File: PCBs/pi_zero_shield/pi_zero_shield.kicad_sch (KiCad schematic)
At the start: 4 parts, among them J1 T1M-10-F-SH-L-K, J3 T1M-06-X-DV

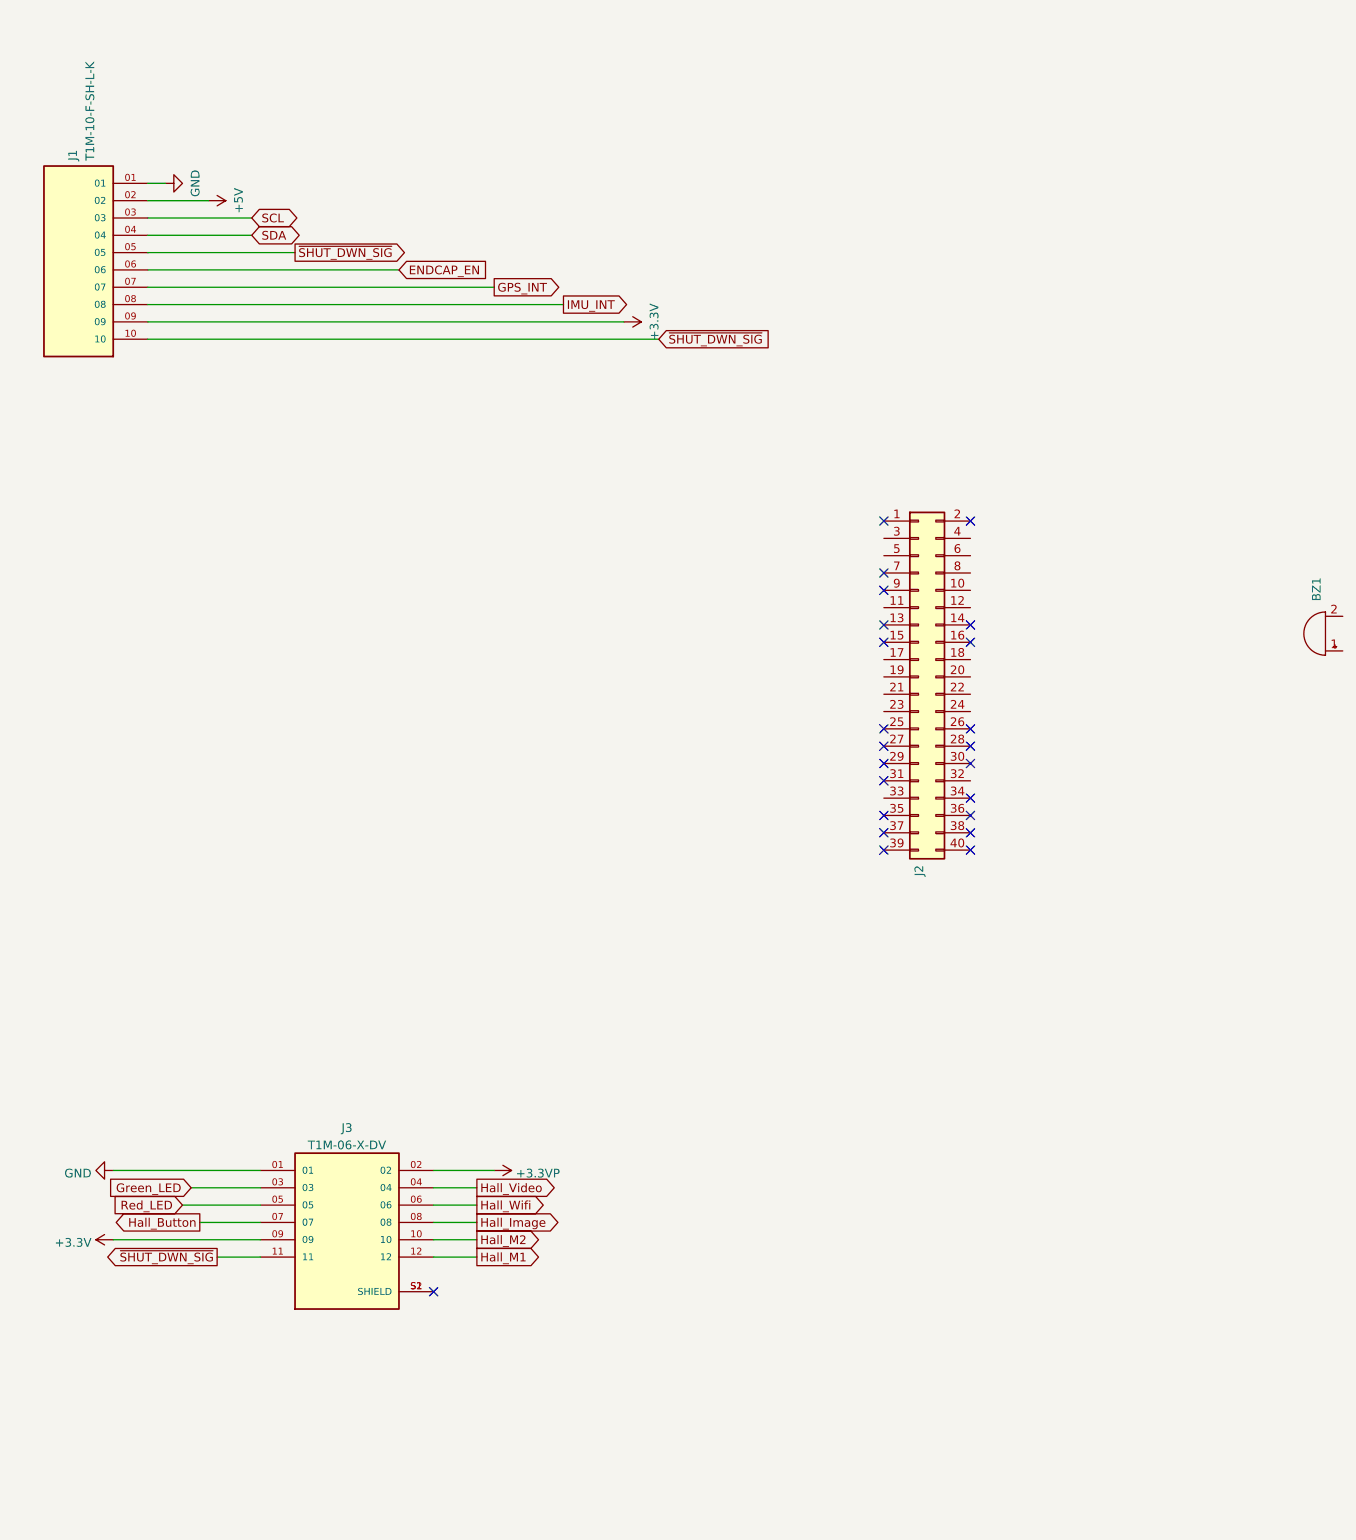
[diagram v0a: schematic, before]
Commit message: number of PCBs for 2nd round of Maka Niu fabrication, in their state after orders made.
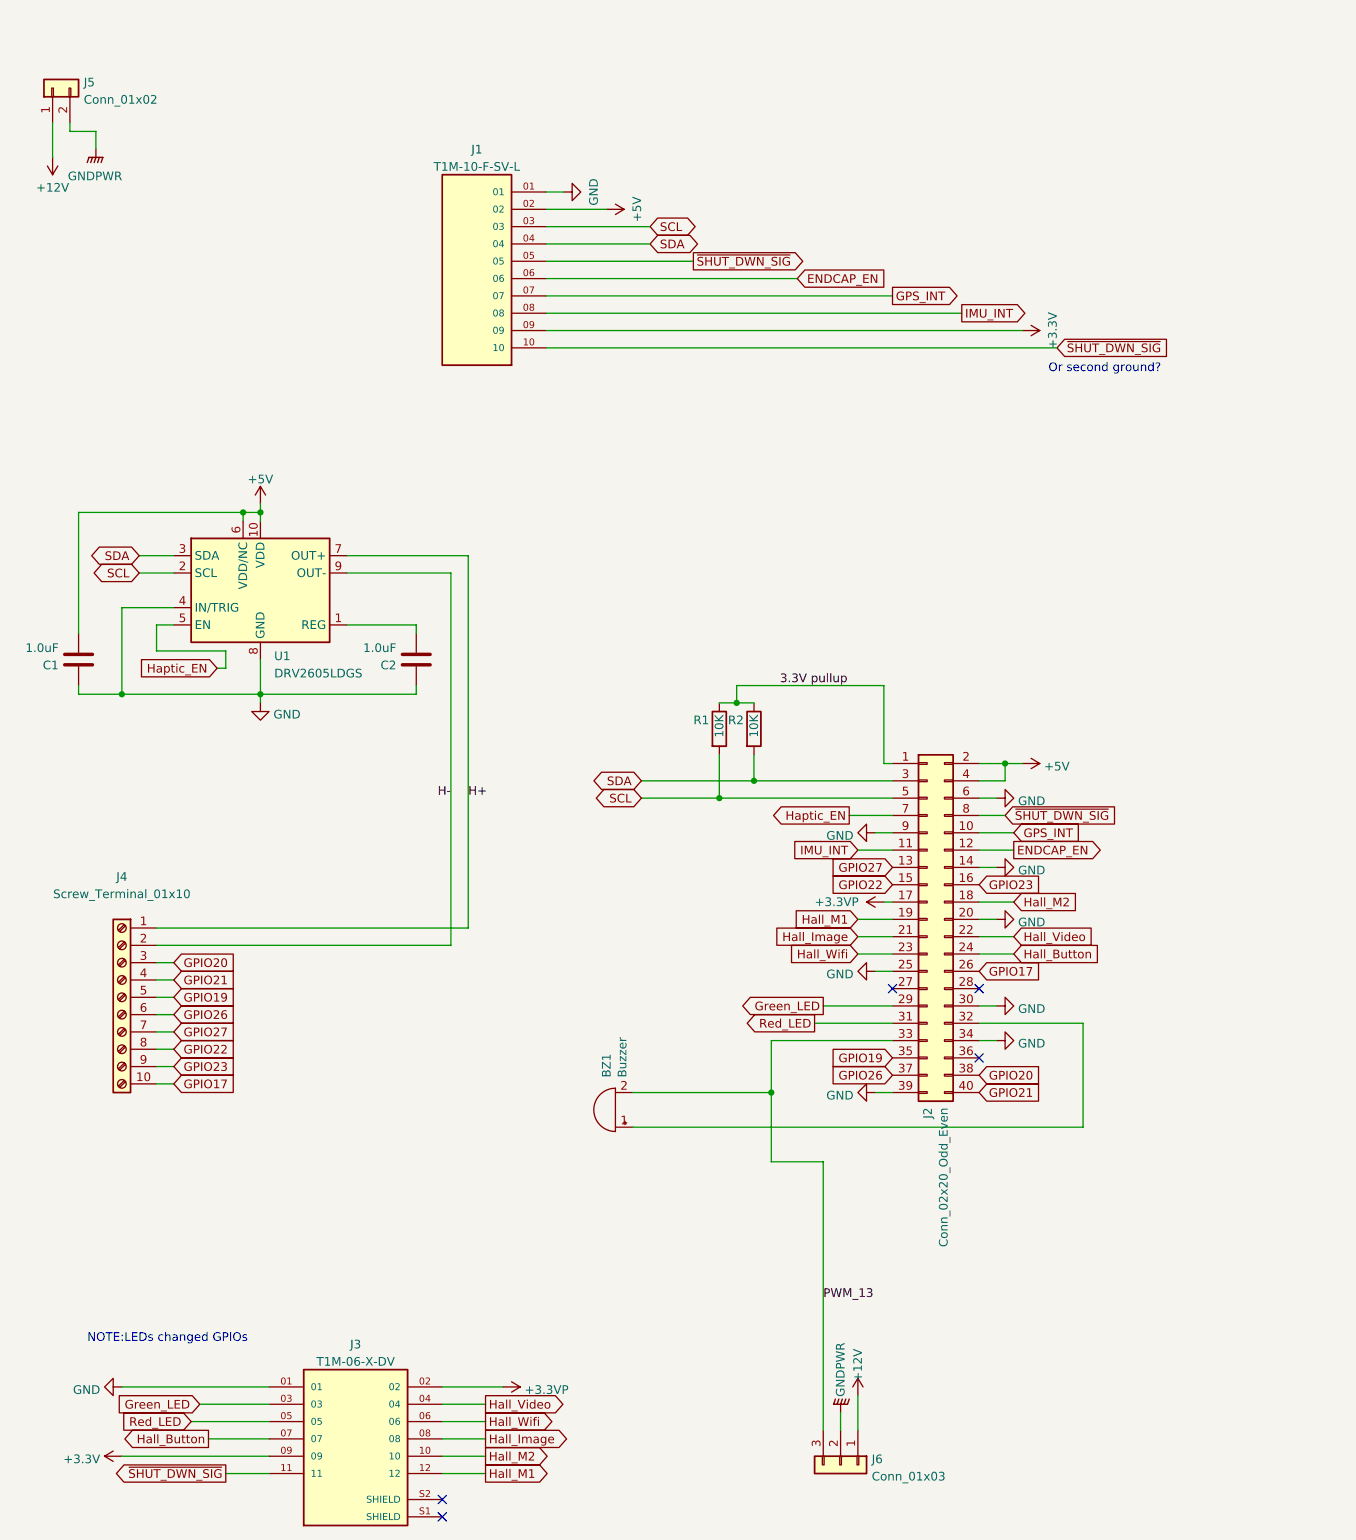
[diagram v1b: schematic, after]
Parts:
- removed J1: T1M-10-F-SH-L-K, custom:SAMTEC_T1M-10-F-SH-L-K, symbol T1M-10-F-SH-L-K:T1M-10-F-SH-L-K
- added C1, C2: 1.0uF, Capacitor_SMD:C_0603_1608Metric, symbol Device:C
- added J1: T1M-10-F-SV-L, SAMTEC_T1M-10-F-SV-L, symbol T1M-10-F-SV-L:T1M-10-F-SV-L
- added J4: Screw_Terminal_01x10, Connector_PinHeader_2.54mm:PinHeader_1x10_P2.54mm_Vertical, symbol Connector:Screw_Terminal_01x10
- added J5: Conn_01x02, Connector_Molex:Molex_Micro-Fit_3.0_43650-0210_1x02-1MP_P3.00mm_Horizontal, symbol Connector_Generic:Conn_01x02
- added J6: Conn_01x03, Connector_Molex:Molex_Micro-Fit_3.0_43650-0310_1x03-1MP_P3.00mm_Horizontal, symbol Connector_Generic:Conn_01x03
- added R1, R2: 10K, Resistor_SMD:R_0603_1608Metric, symbol Device:R
- added U1: DRV2605LDGS, Package_SO:VSSOP-10_3x3mm_P0.5mm, symbol Driver_Haptic:DRV2605LDGS
- BZ1: value (none) -> Buzzer; footprint (none) -> custom:Buzzer_12x9.5RM7.6; Buy Digikey (none) -> skip; Digikey (none) -> 668-1466-ND; LCSC (none) -> C968749
- J2: value (none) -> Conn_02x20_Odd_Even; footprint (none) -> custom:Pi_PinSocket_2x20; Buy Digikey (none) -> Buy; Digikey (none) -> 952-3218-ND
- J3: footprint custom:SAMTEC_T1M-06-X-DV -> SAMTEC_T1M-06-X-DV; Buy Digikey (none) -> skip; Digikey (none) -> -Get from Samtec; MANUFACTURER Samtec -> (none); MAXIMUM_PACKAGE_HEIGHT 6.80mm -> (none); PARTREV B -> (none); STANDARD Manufacturer Recommendations -> (none)
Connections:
- net +3.3VP: now also J2.17 (Pin_17)
- net +3V3: now also J1.09
- net +5V: now also J2.2 (Pin_2), J2.4 (Pin_4), C1.1, J1.02, U1.10 (VDD), U1.6 (VDD/NC)
- net ENDCAP_EN: now also J2.12 (Pin_12), J1.06
- net GND: now also J2.14 (Pin_14), J2.20 (Pin_20), J2.25 (Pin_25), J2.30 (Pin_30), J2.34 (Pin_34), J2.39 (Pin_39), J2.6 (Pin_6), J2.9 (Pin_9), C1.2, C2.2, J1.01, U1.4 (IN/TRIG), U1.8 (GND)
- net GPS_INT: now also J2.10 (Pin_10), J1.07
- net Green_LED: now also J2.29 (Pin_29)
- net Hall_Button: now also J2.24 (Pin_24)
- net Hall_Image: now also J2.21 (Pin_21)
- net Hall_M1: now also J2.19 (Pin_19)
- net Hall_M2: now also J2.18 (Pin_18)
- net Hall_Video: now also J2.22 (Pin_22)
- net Hall_Wifi: now also J2.23 (Pin_23)
- net IMU_INT: now also J2.11 (Pin_11), J1.08
- net Red_LED: now also J2.31 (Pin_31)
- net SCL: now also J2.5 (Pin_5), J1.03, R1.2, U1.2 (SCL)
- net SDA: now also J2.3 (Pin_3), J1.04, R2.2, U1.3 (SDA)
- net ~{SHUT_DWN_SIG}: now also J2.8 (Pin_8), J1.05, J1.10
- net 3.3V pullup: now reaches J2.1 (Pin_1)
- net 3.3V pullup: now also R1.1, R2.1
- net GPIO27: now reaches J2.13 (Pin_13)
- net GPIO27: now also J4.7 (Pin_7)
- net GPIO22: now reaches J2.15 (Pin_15)
- net GPIO22: now also J4.8 (Pin_8)
- net GPIO23: now reaches J2.16 (Pin_16)
- net GPIO23: now also J4.9 (Pin_9)
- net GPIO17: now reaches J2.26 (Pin_26)
- net GPIO17: now also J4.10 (Pin_10)
- net at J2.32 (Pin_32): now also BZ1.1 (-)
- net PWM_13: now reaches J2.33 (Pin_33)
- net PWM_13: now also BZ1.2 (+), J6.3 (Pin_3)
- net GPIO19: now reaches J2.35 (Pin_35)
- net GPIO19: now also J4.5 (Pin_5)
- net GPIO26: now reaches J2.37 (Pin_37)
- net GPIO26: now also J4.6 (Pin_6)
- net GPIO20: now reaches J2.38 (Pin_38)
- net GPIO20: now also J4.3 (Pin_3)
- net GPIO21: now reaches J2.40 (Pin_40)
- net GPIO21: now also J4.4 (Pin_4)
- net Haptic_EN: now reaches J2.7 (Pin_7)
- net Haptic_EN: now also U1.5 (EN)
- net at J3.S1 (SHIELD): no longer J3.S2 (SHIELD)
- new net: C2.1, U1.1 (REG)
- new net +12V: J5.1 (Pin_1), J6.1 (Pin_1)
- new net GNDPWR: J5.2 (Pin_2), J6.2 (Pin_2)
- new net H+: J4.1 (Pin_1), U1.7 (OUT+)
- new net H-: J4.2 (Pin_2), U1.9 (OUT-)
- no-connect marks 23 -> 5
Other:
- note added: "NOTE:LEDs changed GPIOs"
- note added: "Or second ground?"
- moved on the sheet: BZ1, J2
